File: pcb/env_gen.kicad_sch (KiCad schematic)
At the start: 20 parts, among them J9 AudioJack2, SW1 SW_Push, U4 TL074

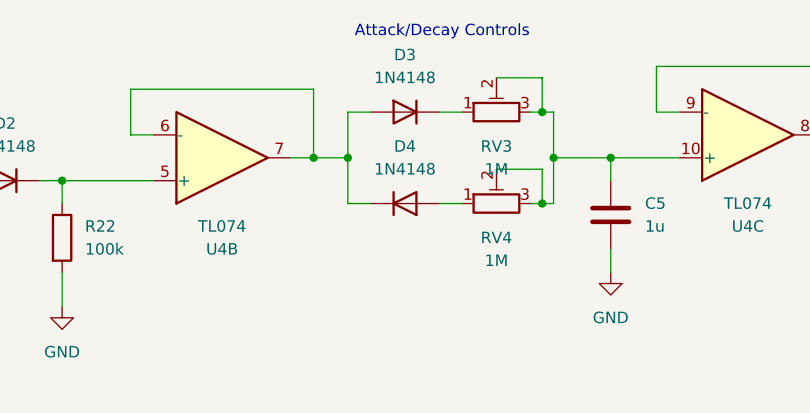
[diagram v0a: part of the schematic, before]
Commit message: update vca
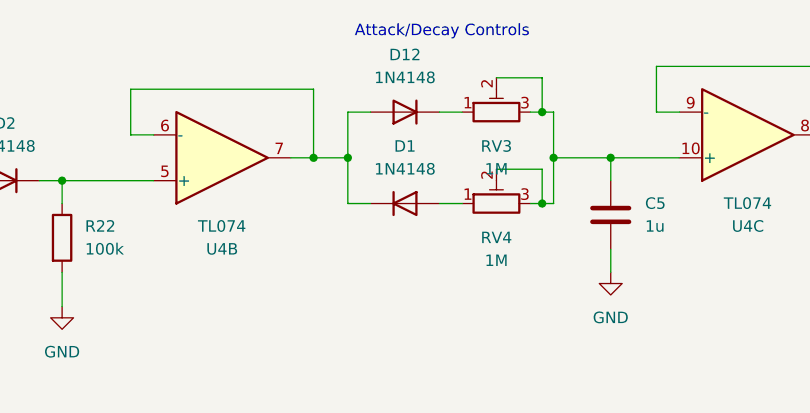
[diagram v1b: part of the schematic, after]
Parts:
- removed D3, D4: 1N4148, Diode_THT:D_DO-35_SOD27_P7.62mm_Horizontal, symbol Diode:1N4148
- added D1, D12: 1N4148, Diode_THT:D_DO-35_SOD27_P7.62mm_Horizontal, symbol Diode:1N4148
- C16, C17, C18, C5: footprint (none) -> Capacitor_THT:C_Disc_D6.0mm_W2.5mm_P5.00mm
- J9: footprint (none) -> Connector_Audio:Jack_3.5mm_CUI_SJ1-3513N_Horizontal
- R20, R21, R22, R23, R30, R31, R32, R33: footprint (none) -> Resistor_THT:R_Axial_DIN0207_L6.3mm_D2.5mm_P10.16mm_Horizontal
- RV3, RV4: footprint (none) -> Potentiometer_THT:Potentiometer_Bourns_PTV09A-1_Single_Vertical
- SW1: footprint (none) -> Button_Switch_Keyboard:SW_Cherry_MX_1.00u_PCB
- U4: footprint (none) -> Package_DIP:DIP-14_W7.62mm
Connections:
- net at U4.6 (-), U4.7: now also D1.1 (K), D12.2 (A)
- net at RV4.1: now also D1.2 (A)
- net at RV3.1: now also D12.1 (K)
